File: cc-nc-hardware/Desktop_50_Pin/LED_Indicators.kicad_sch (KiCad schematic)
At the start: 7 parts, among them J5 Conn_01x03_Male, U8 74HC14

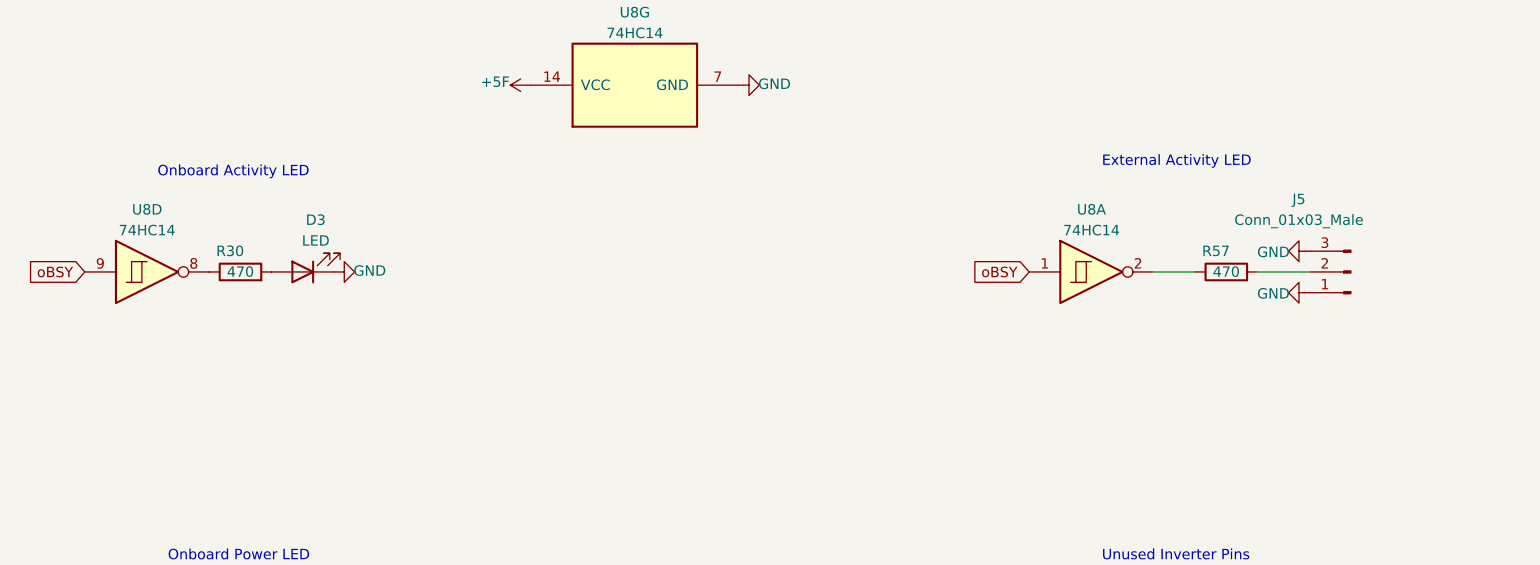
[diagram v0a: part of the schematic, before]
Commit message: Desktop PCB Version 2023.03a
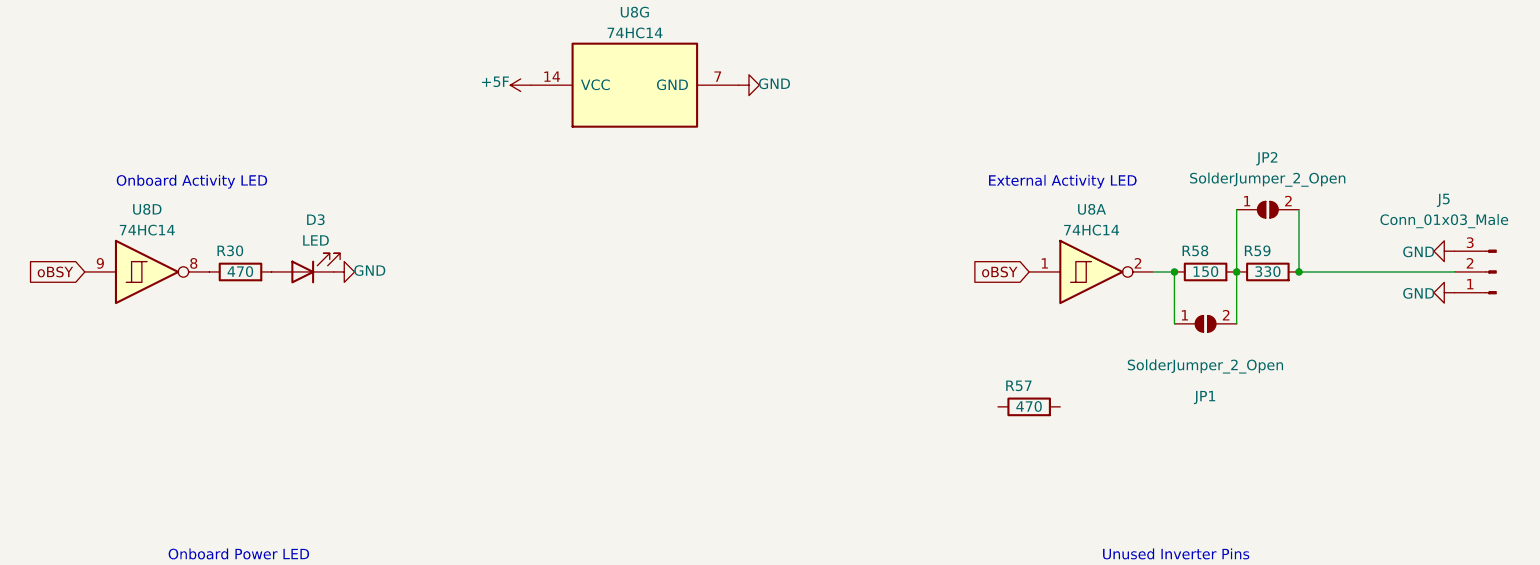
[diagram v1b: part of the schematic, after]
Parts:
- added JP1, JP2: SolderJumper_2_Open, Jumper:SolderJumper-2_P1.3mm_Open_RoundedPad1.0x1.5mm, symbol Jumper:SolderJumper_2_Open
- added R58: 150, Resistor_SMD:R_0603_1608Metric_Pad0.98x0.95mm_HandSolder, symbol Device:R
- added R59: 330, Resistor_SMD:R_0603_1608Metric_Pad0.98x0.95mm_HandSolder, symbol Device:R
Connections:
- net at U8.2: now also JP1.1 (A), R58.1; no longer R57.1
- net at J5.2 (Pin_2): now also JP2.2 (B), R59.2; no longer R57.2
- new net: JP1.2 (B), JP2.1 (A), R58.2, R59.1
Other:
- moved on the sheet: J5, R57
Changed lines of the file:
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@@
 (kicad_sch (version 20211123) (generator eeschema)
   (paper "A4")
-  (wire (pts (xy 223.52 60.96) (xy 217.17 60.96))
-    (stroke (width 0) (type default) (color 0 0 0 0))
-  )
-  (wire (pts (xy 209.55 60.96) (xy 204.47 60.96))
+  (junction (at 214.63 60.96) (diameter 0) (color 0 0 0 0)
+  )
+  (junction (at 222.25 60.96) (diameter 0) (color 0 0 0 0)
+  )
+  (junction (at 207.01 60.96) (diameter 0) (color 0 0 0 0)
+  )
+  (wire (pts (xy 222.25 60.96) (xy 241.3 60.96))
+    (stroke (width 0) (type default) (color 0 0 0 0))
+  )
+  (wire (pts (xy 214.63 53.34) (xy 214.63 60.96))
+    (stroke (width 0) (type default) (color 0 0 0 0))
+  )
+  (wire (pts (xy 204.47 60.96) (xy 207.01 60.96))
+    (stroke (width 0) (type default) (color 0 0 0 0))
+  )
+  (wire (pts (xy 222.25 53.34) (xy 222.25 60.96))
+    (stroke (width 0) (type default) (color 0 0 0 0))
+  )
+  (wire (pts (xy 214.63 60.96) (xy 214.63 67.31))
+    (stroke (width 0) (type default) (color 0 0 0 0))
+  )
+  (wire (pts (xy 207.01 60.96) (xy 207.01 67.31))
     (stroke (width 0) (type default) (color 0 0 0 0))
   )
@@
     (effects (font (size 1.27 1.27)) (justify left bottom))
   )
-  (text "Onboard Activity LED" (at 82.55 49.53 0)
+  (text "Onboard Activity LED" (at 77.47 50.8 0)
     (effects (font (size 1.27 1.27)) (justify left bottom))
   )
-  (text "External Activity LED" (at 198.12 48.26 0)
+  (text "External Activity LED" (at 184.15 50.8 0)
     (effects (font (size 1.27 1.27)) (justify left bottom))
   )
@@
     )
   )
+  (symbol (lib_id "Device:R") (at 218.44 60.96 90) (unit 1)
+    (in_bom yes) (on_board yes)
+    (property "Reference" "R59" (id 0) (at 217.17 58.42 90))
+    (property "Value" "330" (id 1) (at 218.44 60.96 90))
+    (property "Footprint" "Resistor_SMD:R_0603_1608Metric_Pad0.98x0.95mm_HandSolder" (id 2) (at 218.44 62.738 90)
+      (effects (font (size 1.27 1.27)) hide)
+    )
+    (property "Datasheet" "~" (id 3) (at 218.44 60.96 0)
+      (effects (font (size 1.27 1.27)) hide)
+    )
+    (pin "1")
+    (pin "2")
+  )
   (symbol (lib_id "power:GND") (at 153.67 38.1 90) (unit 1)
     (in_bom yes) (on_board yes)
@@
     )
     (pin "1")
+  )
+  (symbol (lib_id "Device:R") (at 210.82 60.96 90) (unit 1)
+    (in_bom yes) (on_board yes)
+    (property "Reference" "R58" (id 0) (at 209.55 58.42 90))
+    (property "Value" "150" (id 1) (at 210.82 60.96 90))
+    (property "Footprint" "Resistor_SMD:R_0603_1608Metric_Pad0.98x0.95mm_HandSolder" (id 2) (at 210.82 62.738 90)
+      (effects (font (size 1.27 1.27)) hide)
+    )
+    (property "Datasheet" "~" (id 3) (at 210.82 60.96 0)
+      (effects (font (size 1.27 1.27)) hide)
+    )
+    (pin "1")
+    (pin "2")
   )
   (symbol (lib_id "74xx:74HC14") (at 81.28 60.96 0) (unit 4)
@@
     (pin "1")
   )
-  (symbol (lib_id "power:GND") (at 223.52 63.5 270) (unit 1)
-    (in_bom yes) (on_board yes)
-    (property "Reference" "#PWR069" (id 0) (at 217.17 63.5 0)
-      (effects (font (size 1.27 1.27)) hide)
-    )
-    (property "Value" "GND" (id 1) (at 219.1258 63.627 90))
-    (property "Footprint" "" (id 2) (at 223.52 63.5 0)
-      (effects (font (size 1.27 1.27)) hide)
-    )
-    (property "Datasheet" "" (id 3) (at 223.52 63.5 0)
+  (symbol (lib_id "Jumper:SolderJumper_2_Open") (at 210.82 67.31 0) (unit 1)
+    (in_bom yes) (on_board yes)
+    (property "Reference" "JP1" (id 0) (at 210.82 76.2 0))
+    (property "Value" "SolderJumper_2_Open" (id 1) (at 210.82 72.39 0))
+    (property "Footprint" "Jumper:SolderJumper-2_P1.3mm_Open_RoundedPad1.0x1.5mm" (id 2) (at 210.82 67.31 0)
+      (effects (font (size 1.27 1.27)) hide)
+    )
+    (property "Datasheet" "~" (id 3) (at 210.82 67.31 0)
+      (effects (font (size 1.27 1.27)) hide)
+    )
+    (pin "1")
+    (pin "2")
+  )
+  (symbol (lib_id "Jumper:SolderJumper_2_Open") (at 218.44 53.34 0) (unit 1)
+    (in_bom yes) (on_board yes) (fields_autoplaced)
+    (property "Reference" "JP2" (id 0) (at 218.44 46.99 0))
+    (property "Value" "SolderJumper_2_Open" (id 1) (at 218.44 49.53 0))
+    (property "Footprint" "Jumper:SolderJumper-2_P1.3mm_Open_RoundedPad1.0x1.5mm" (id 2) (at 218.44 53.34 0)
+      (effects (font (size 1.27 1.27)) hide)
+    )
+    (property "Datasheet" "~" (id 3) (at 218.44 53.34 0)
+      (effects (font (size 1.27 1.27)) hide)
+    )
+    (pin "1")
+    (pin "2")
+  )
+  (symbol (lib_id "power:GND") (at 241.3 63.5 270) (unit 1)
+    (in_bom yes) (on_board yes)
+    (property "Reference" "#PWR069" (id 0) (at 234.95 63.5 0)
+      (effects (font (size 1.27 1.27)) hide)
+    )
+    (property "Value" "GND" (id 1) (at 236.9058 63.627 90))
+    (property "Footprint" "" (id 2) (at 241.3 63.5 0)
+      (effects (font (size 1.27 1.27)) hide)
+    )
+    (property "Datasheet" "" (id 3) (at 241.3 63.5 0)
       (effects (font (size 1.27 1.27)) hide)
     )
@@
     (pin "2")
   )
-  (symbol (lib_id "Connector:Conn_01x03_Male") (at 228.6 60.96 180) (unit 1)
-    (in_bom yes) (on_board yes)
-    (property "Reference" "J5" (id 0) (at 222.25 52.07 0))
-    (property "Value" "Conn_01x03_Male" (id 1) (at 222.25 54.61 0))
-    (property "Footprint" "Connector_PinHeader_2.54mm:PinHeader_1x03_P2.54mm_Vertical" (id 2) (at 228.6 60.96 0)
-      (effects (font (size 1.27 1.27)) hide)
-    )
-    (property "Datasheet" "~" (id 3) (at 228.6 60.96 0)
+  (symbol (lib_id "Connector:Conn_01x03_Male") (at 246.38 60.96 180) (unit 1)
+    (in_bom yes) (on_board yes)
+    (property "Reference" "J5" (id 0) (at 240.03 52.07 0))
+    (property "Value" "Conn_01x03_Male" (id 1) (at 240.03 54.61 0))
+    (property "Footprint" "Connector_PinHeader_2.54mm:PinHeader_1x03_P2.54mm_Vertical" (id 2) (at 246.38 60.96 0)
+      (effects (font (size 1.27 1.27)) hide)
+    )
+    (property "Datasheet" "~" (id 3) (at 246.38 60.96 0)
       (effects (font (size 1.27 1.27)) hide)
     )
@@
     (pin "1")
   )
-  (symbol (lib_id "Device:R") (at 213.36 60.96 90) (unit 1)
-    (in_bom yes) (on_board yes)
-    (property "Reference" "R57" (id 0) (at 212.09 58.42 90))
-    (property "Value" "470" (id 1) (at 213.36 60.96 90))
-    (property "Footprint" "Resistor_SMD:R_0402_1005Metric_Pad0.72x0.64mm_HandSolder" (id 2) (at 213.36 62.738 90)
-      (effects (font (size 1.27 1.27)) hide)
-    )
-    (property "Datasheet" "~" (id 3) (at 213.36 60.96 0)
+  (symbol (lib_id "Device:R") (at 189.23 77.47 90) (unit 1)
+    (in_bom yes) (on_board yes)
+    (property "Reference" "R57" (id 0) (at 187.96 74.93 90))
+    (property "Value" "470" (id 1) (at 189.23 77.47 90))
+    (property "Footprint" "Resistor_SMD:R_0402_1005Metric_Pad0.72x0.64mm_HandSolder" (id 2) (at 189.23 79.248 90)
+      (effects (font (size 1.27 1.27)) hide)
+    )
+    (property "Datasheet" "~" (id 3) (at 189.23 77.47 0)
       (effects (font (size 1.27 1.27)) hide)
     )
@@
     (pin "7")
   )
-  (symbol (lib_id "power:GND") (at 223.52 58.42 270) (unit 1)
-    (in_bom yes) (on_board yes)
-    (property "Reference" "#PWR068" (id 0) (at 217.17 58.42 0)
-      (effects (font (size 1.27 1.27)) hide)
-    )
-    (property "Value" "GND" (id 1) (at 219.1258 58.547 90))
-    (property "Footprint" "" (id 2) (at 223.52 58.42 0)
-      (effects (font (size 1.27 1.27)) hide)
-    )
-    (property "Datasheet" "" (id 3) (at 223.52 58.42 0)
-      (effects (font (size 1.27 1.27)) hide)
-    )
+  (symbol (lib_id "power:GND") (at 241.3 58.42 270) (unit 1)
+    (in_bom yes) (on_board yes)
+    (property "Reference" "#PWR068" (id 0) (at 234.95 58.42 0)
+      (effects (font (size 1.27 1.27)) hide)
+    )
+    (property "Value" "GND" (id 1) (at 236.9058 58.547 90))
+    (property "Footprint" "" (id 2) (at 241.3 58.42 0)
+      (effects (font (size 1.27 1.27)) hide)
+    )
+    (property "Datasheet" "" (id 3) (at 241.3 58.42 0)
+      (effects (font (size 1.27 1.27)) hide)
+    )

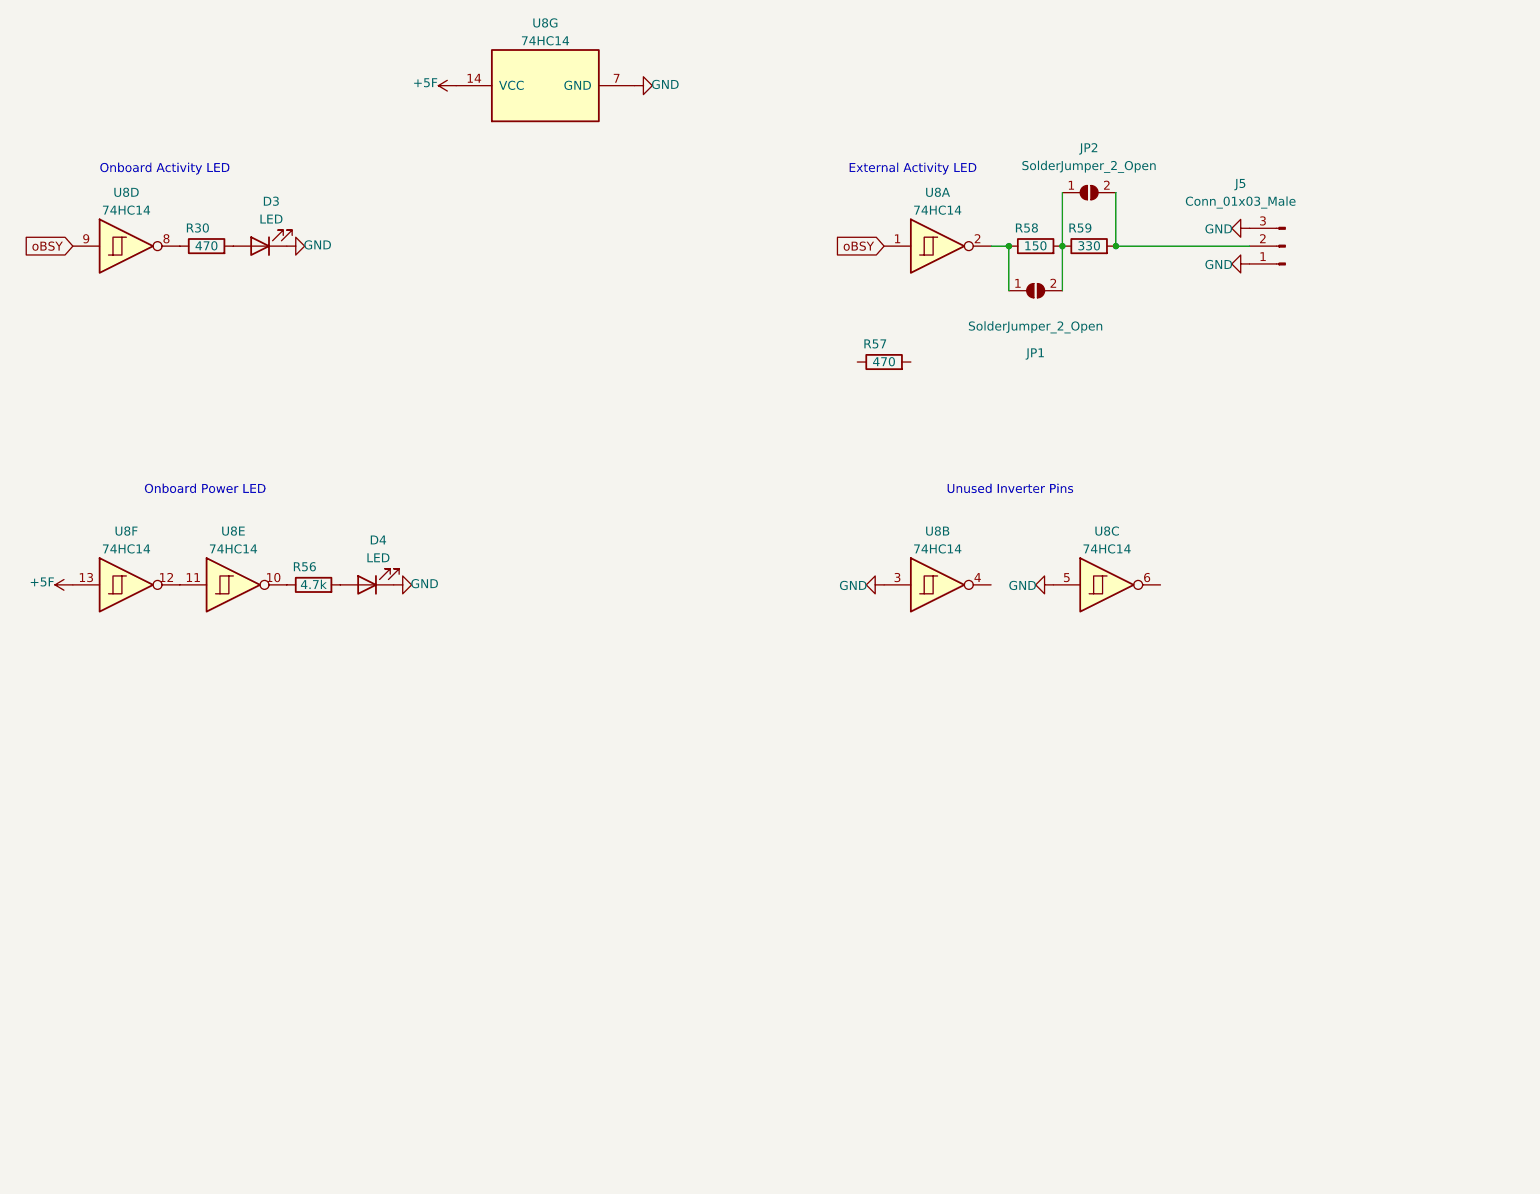
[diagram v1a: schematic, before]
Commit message: Desktop 2023.09a Hardware Design
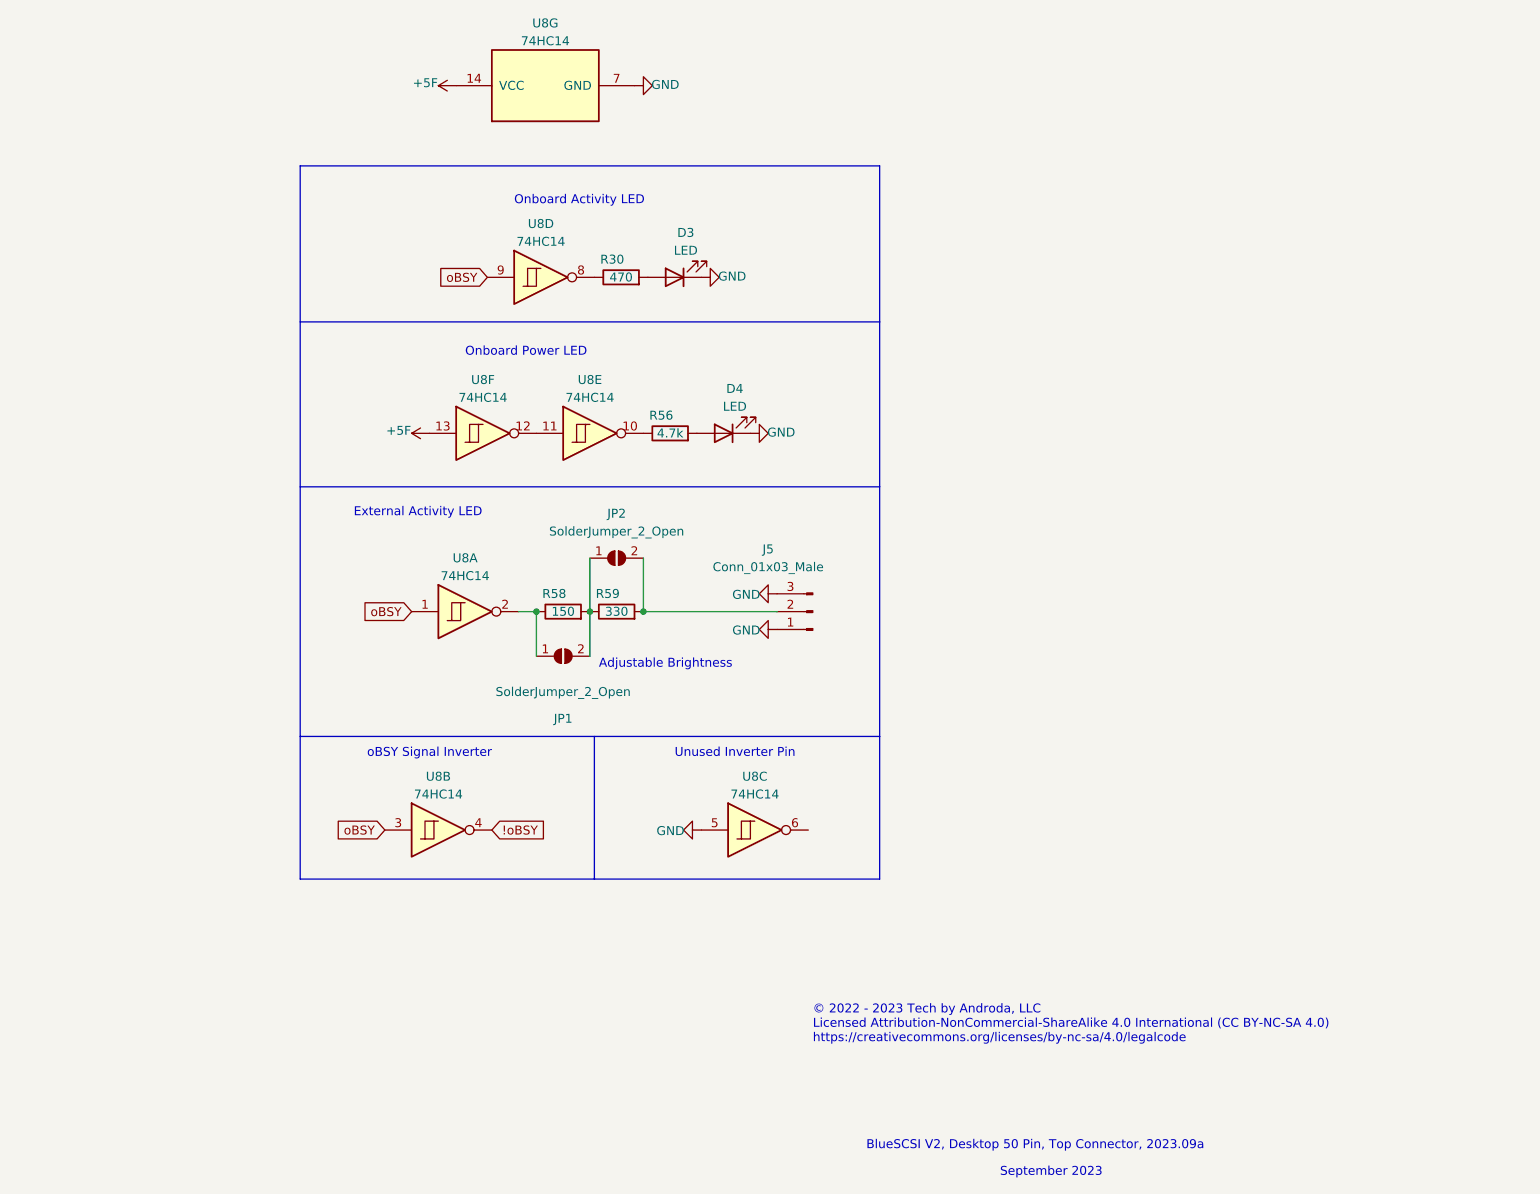
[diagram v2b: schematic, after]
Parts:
- removed R57: 470, Resistor_SMD:R_0402_1005Metric_Pad0.72x0.64mm_HandSolder, symbol Device:R
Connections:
- net GND: no longer U8.3
- net oBSY: now also U8.3
- net !oBSY: now reaches U8.4
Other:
- note added: "Adjustable Brightness"
- note added: "BlueSCSI V2, Desktop 50 Pin, Top Connector, 2023.09a"
- note added: "September 2023"
- note added: "Unused Inverter Pin"
- note added: "oBSY Signal Inverter"
- note added: "© 2022 - 2023 Tech by Androda, LLC Licensed Attribution-NonCommercial-ShareAlike 4.0 International (CC BY-NC-SA 4.0) https://creativecommons.org/licenses/by-nc-sa/4.0/legalcode"
- note removed: "Unused Inverter Pins"
- moved on the sheet: D3, D4, J5, JP1, JP2, R30, R56, R58, R59, U8A, U8B, U8C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
